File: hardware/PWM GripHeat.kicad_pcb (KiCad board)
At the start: 2 copper layers, 54.5 x 29.5 mm, 56 parts, among them J1 1770885, J2 Screw_Terminal_01x08, U1 ATtiny85-20P, U2 SiA462DJ, U3 LM324

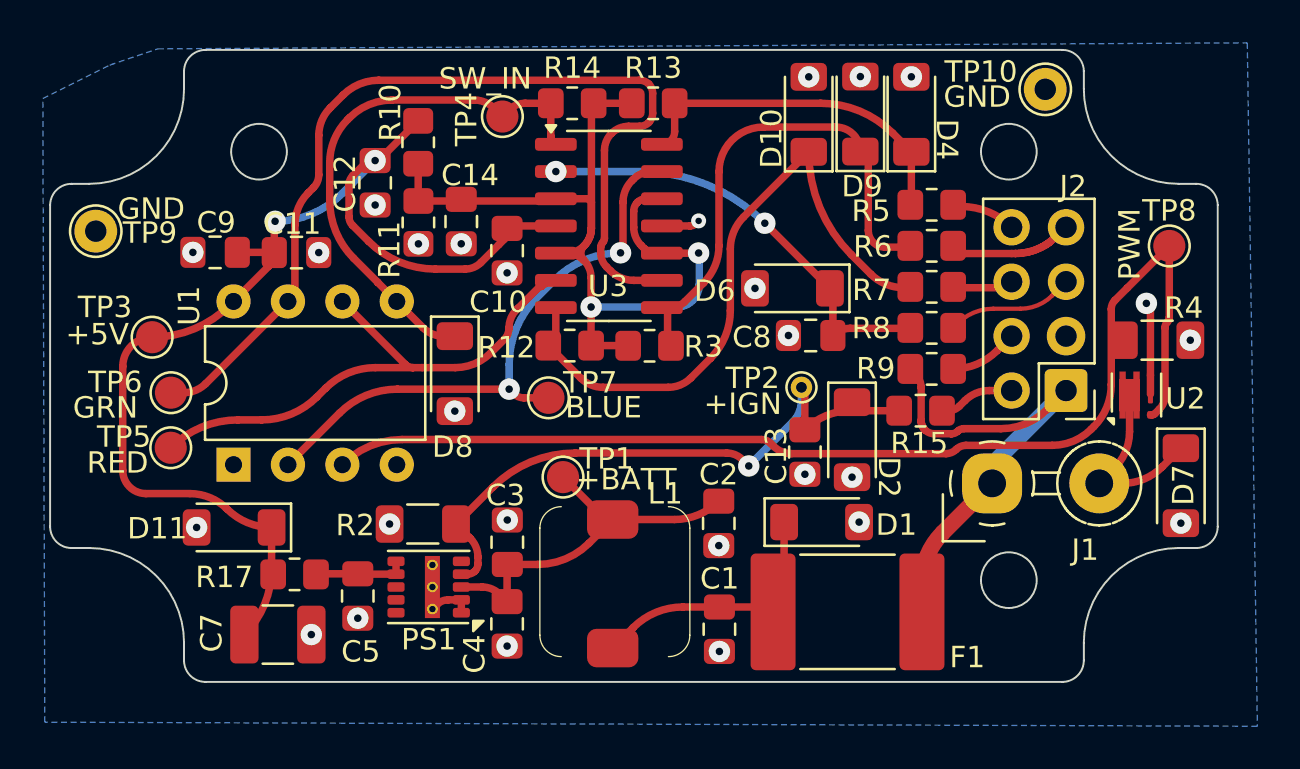
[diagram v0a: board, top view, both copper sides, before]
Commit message: Released
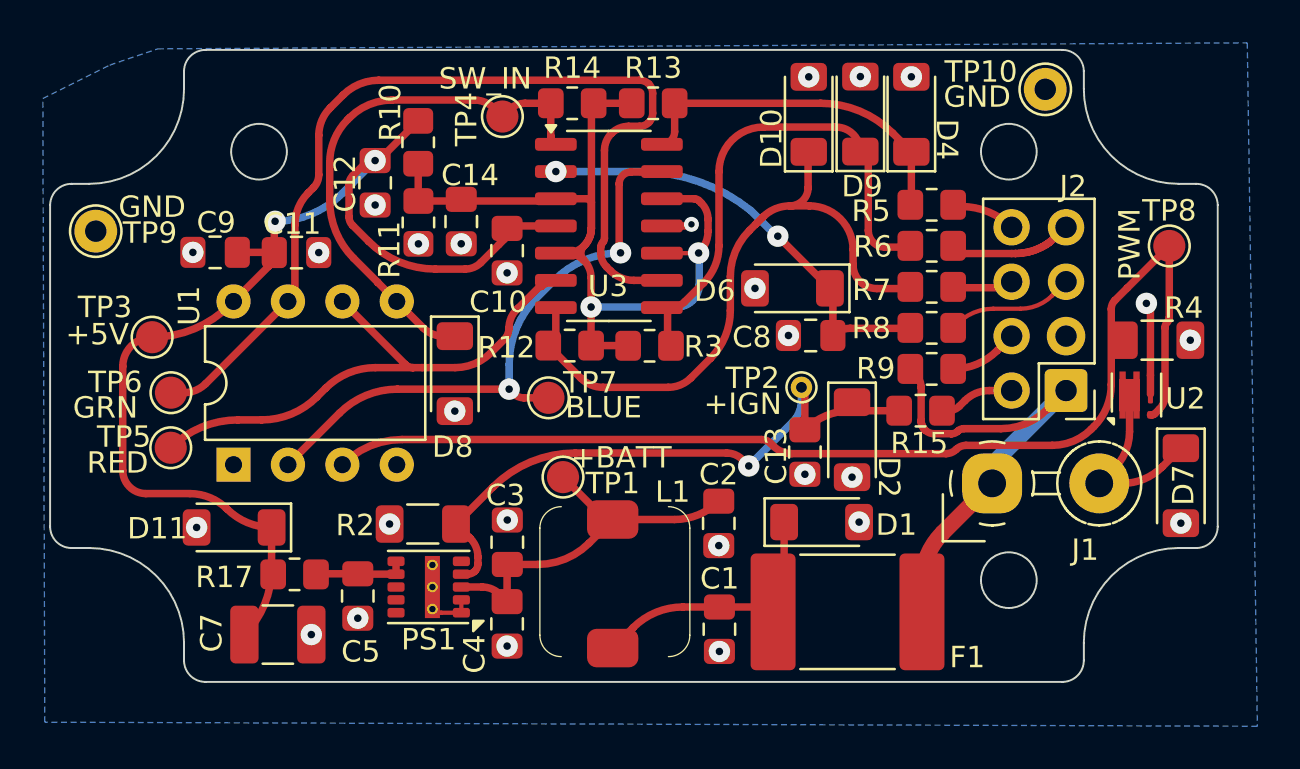
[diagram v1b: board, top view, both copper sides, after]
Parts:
- moved G*** 0.30 mm to (151.0, 101.3)
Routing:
- net /BLU: track 27.8 -> 28.4 mm
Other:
- rule pad_to_mask_clearance: 0 -> 0.0508
- board text added: "Epoxy"
- board text added: "FR4 natural"
- board text added: "Purple"
- board text added: "White"
